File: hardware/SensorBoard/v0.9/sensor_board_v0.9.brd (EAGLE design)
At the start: 52.5 x 43 mm, 43 parts, among them IC1 BMP280, IC2 VREF, J3 USB-MICROB, U1 LMP91000, U10 CCS811, U11 RFM69HW, U2 TSL2561, U3 ATMEGA328P-MU, U7 SHT31, U8 MCP1703/3.3V, Y1 16MHZ

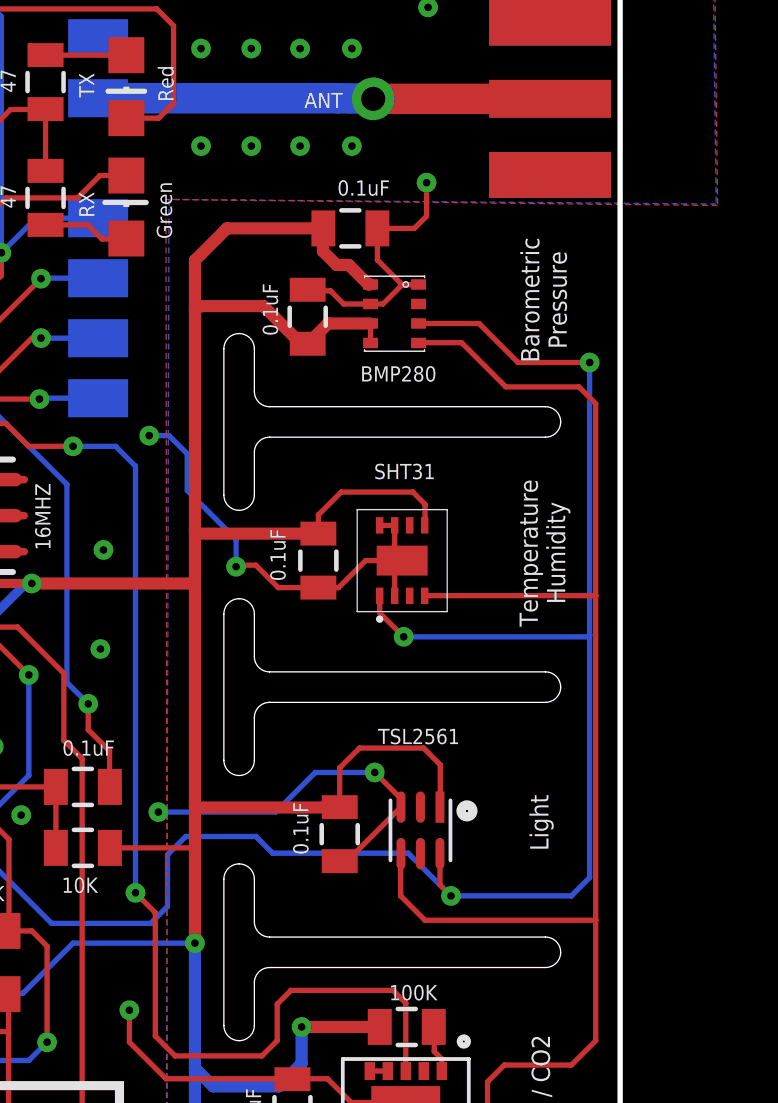
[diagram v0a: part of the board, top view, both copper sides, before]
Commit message: Minor component adjustments
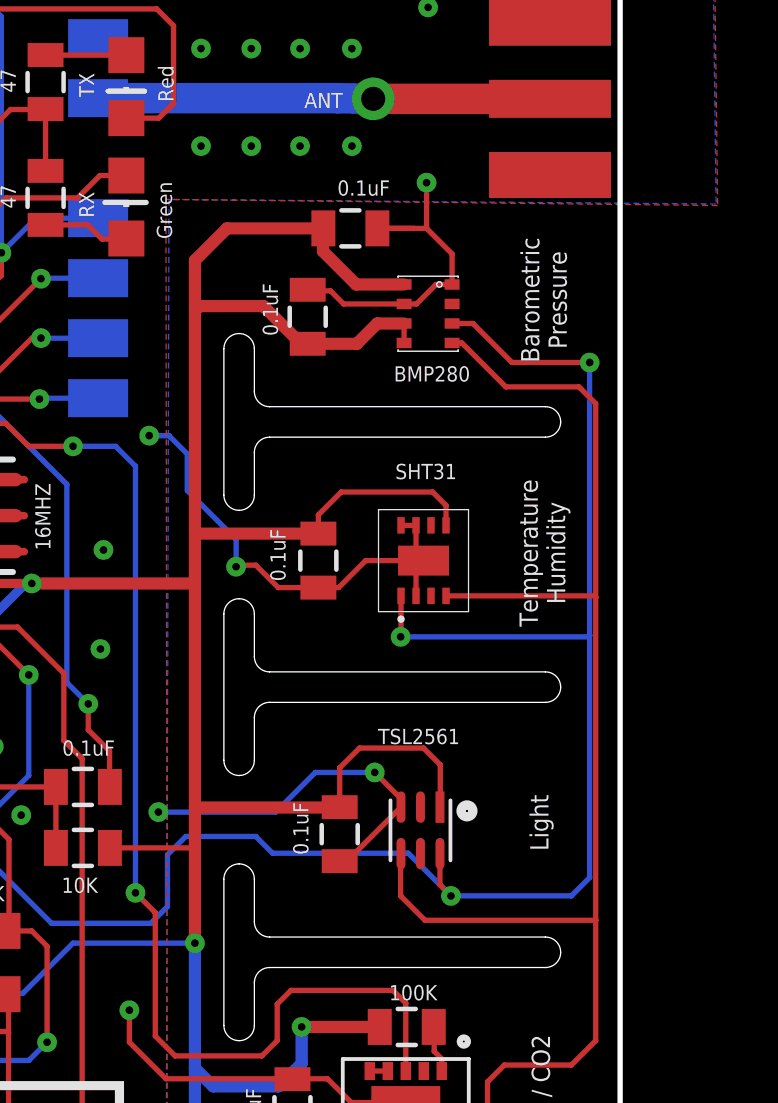
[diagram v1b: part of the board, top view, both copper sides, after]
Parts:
- moved IC1 1.12 mm to (49.5, 35.6)
- moved U7 0.71 mm to (49.4, 27.4)
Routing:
- net GND: track 52.8 -> 56.1 mm
- net VCC: track 166.3 -> 169.2 mm
- net SCL: track 96.0 -> 94.2 mm
- net SDA: track 98.8 -> 97.5 mm
